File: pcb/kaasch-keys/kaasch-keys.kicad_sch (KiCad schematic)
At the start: 62 parts, among them SW1 SW_Push, SW10 SW_Push, SW11 SW_Push, SW12 SW_Push, SW13 SW_Push, SW14 SW_Push, SW15 SW_Push, SW16 SW_Push, SW17 SW_Push, SW18 SW_Push, SW19 SW_Push, SW2 SW_Push, SW20 SW_Push, SW21 SW_Push, SW22 SW_Push, SW23 SW_Push, SW24 SW_Push, SW25 SW_Push, SW26 SW_Push, SW27 SW_Push, SW28 SW_Push, SW29 SW_Push, SW3 SW_Push, SW30 SW_Push, SW4 SW_Push, SW5 SW_Push, SW6 SW_Push, SW7 SW_Push, SW8 SW_Push, SW9 SW_Push

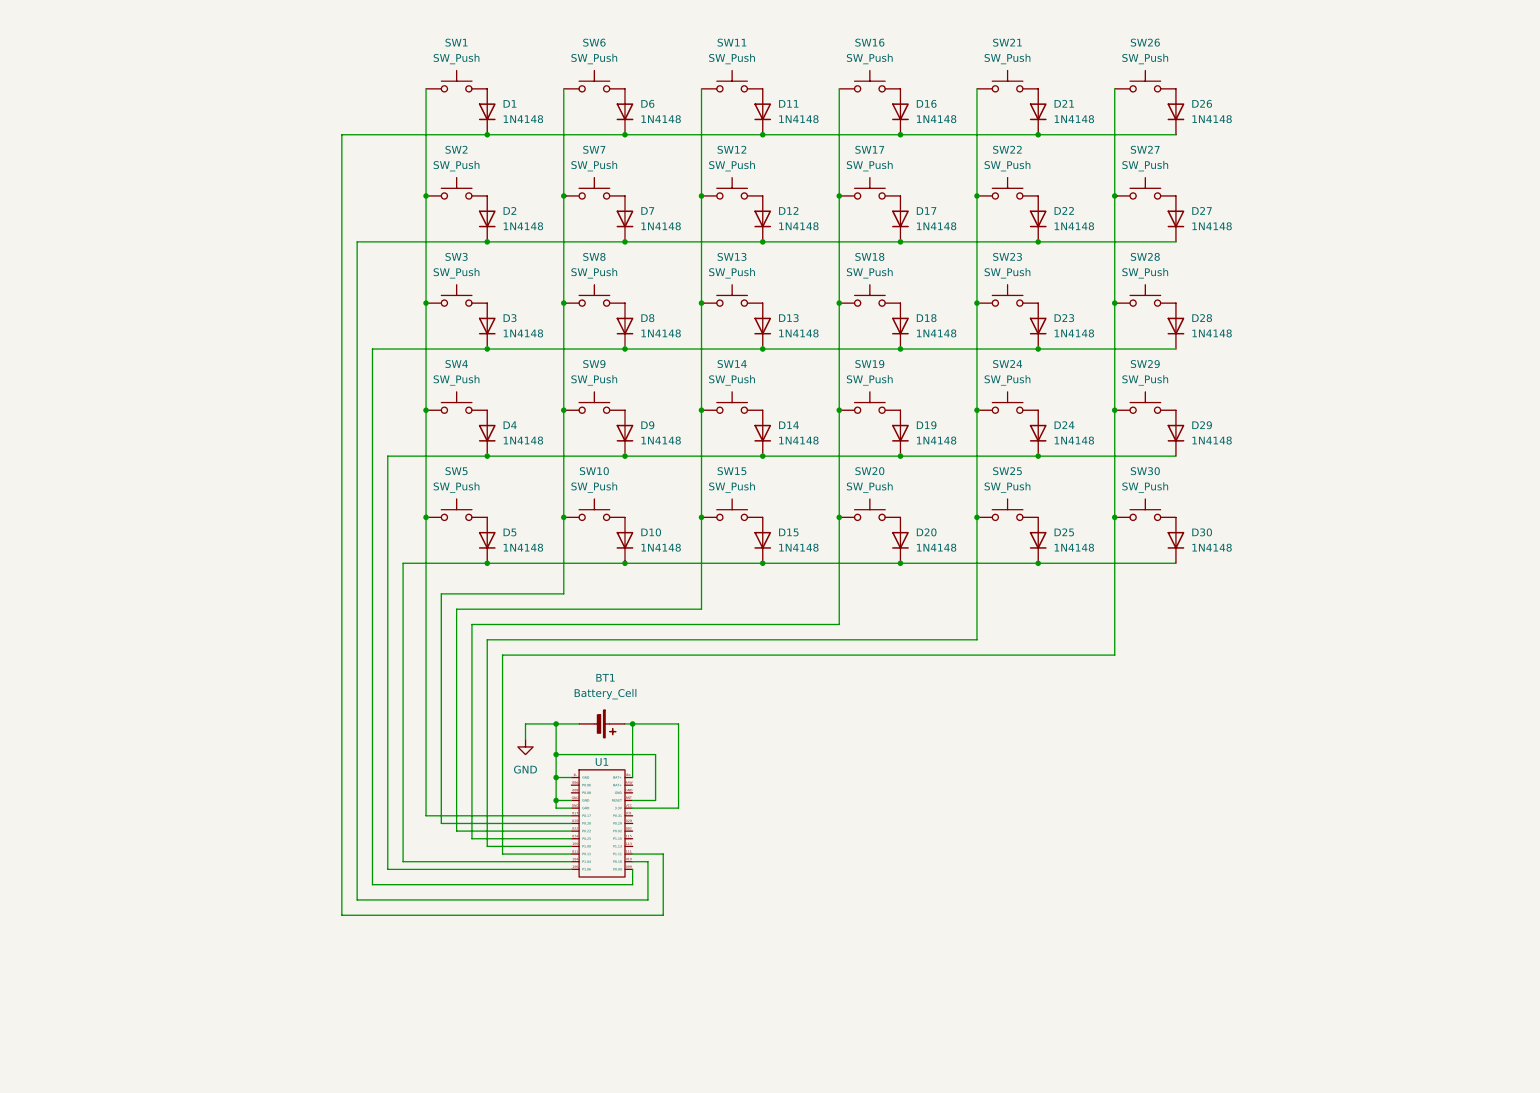
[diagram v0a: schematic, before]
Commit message: lets goo
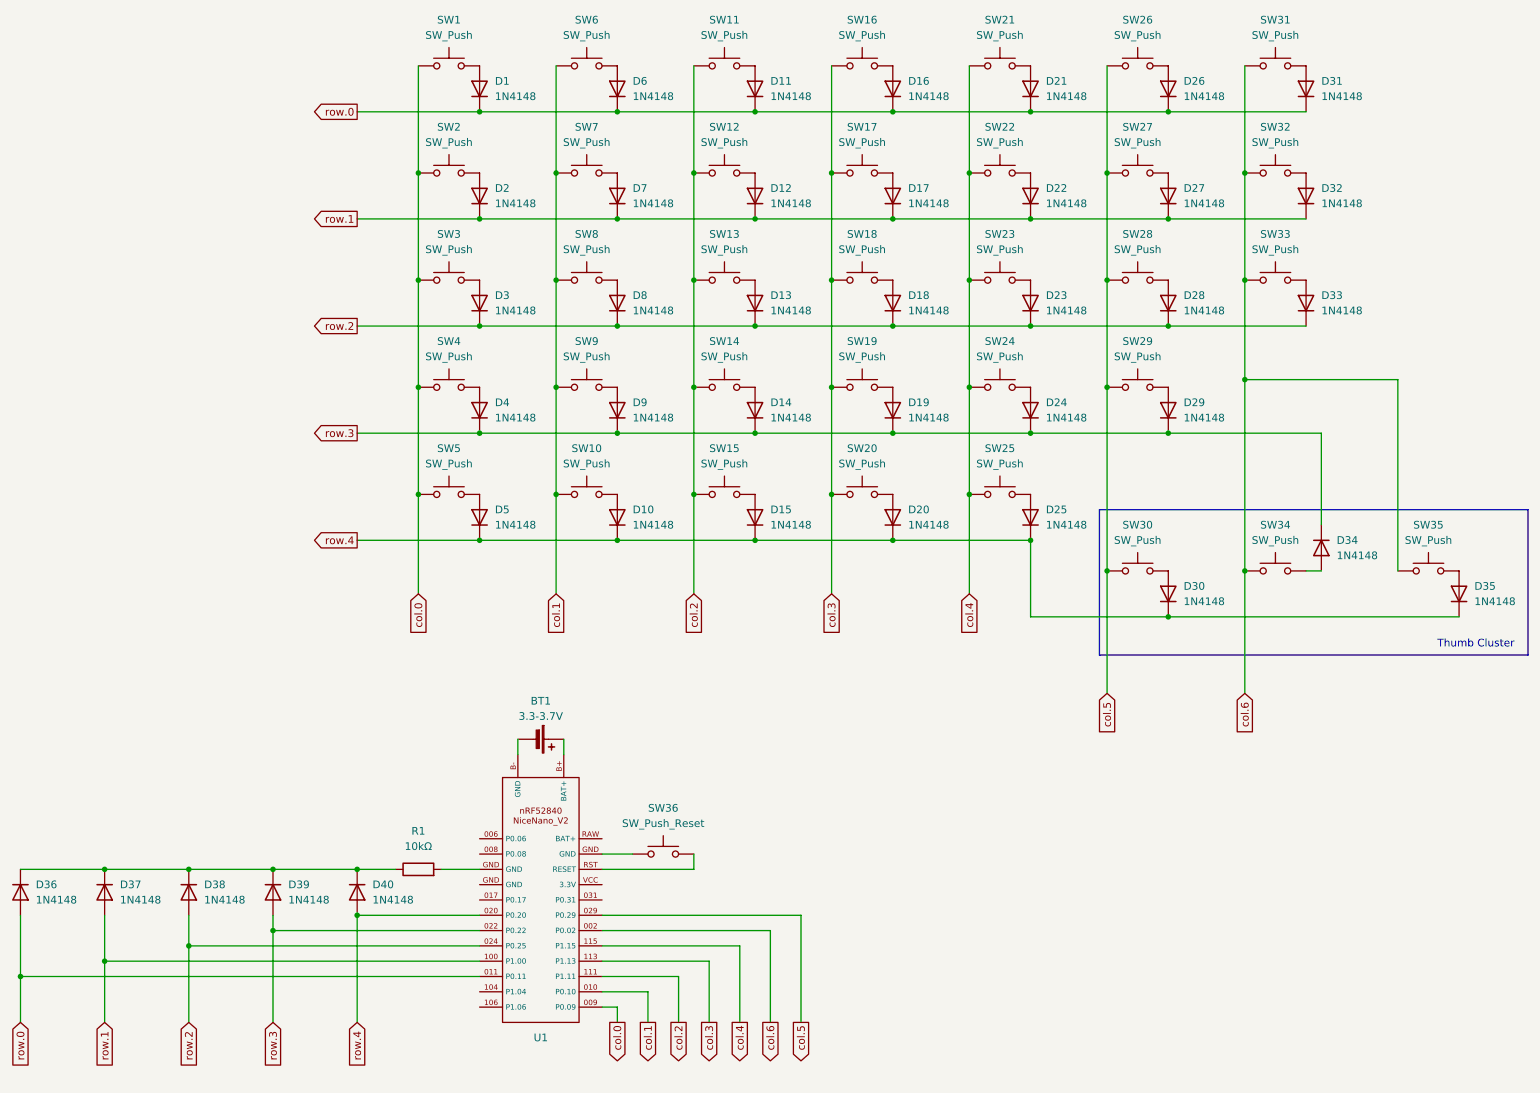
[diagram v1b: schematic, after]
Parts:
- added D31, D32, D33, D34, D35, D36, D37, D38, D39, D40: 1N4148, Diode_THT:D_DO-35_SOD27_P7.62mm_Horizontal, symbol Diode:1N4148
- added R1: 10kΩ, symbol Device:R
- added SW31, SW32, SW33, SW34, SW35: SW_Push, symbol Switch:SW_Push
- added SW36: SW_Push_Reset, symbol Switch:SW_Push
- BT1: value Battery_Cell -> 3.3-3.7V
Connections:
- net col.0: now reaches SW1.1, SW2.1, SW3.1, SW4.1, SW5.1
- net col.0: now also U1.009 (P0.09); no longer U1.017 (P0.17)
- net row.3: now reaches D14.1 (K), D19.1 (K), D24.1 (K), D29.1 (K), D4.1 (K), D9.1 (K)
- net row.3: now also U1.022 (P0.22), D34.1 (K), D39.2 (A); no longer U1.106 (P1.06)
- net row.4: now reaches D10.1 (K), D15.1 (K), D20.1 (K), D25.1 (K), D30.1 (K), D5.1 (K)
- net row.4: now also U1.020 (P0.20), D35.1 (K), D40.2 (A); no longer U1.104 (P1.04)
- net row.2: now reaches D13.1 (K), D18.1 (K), D23.1 (K), D28.1 (K), D3.1 (K), D8.1 (K)
- net row.2: now also U1.024 (P0.25), D33.1 (K), D38.2 (A); no longer U1.009 (P0.09)
- net col.2: now reaches SW11.1, SW12.1, SW13.1, SW14.1, SW15.1
- net col.2: now also U1.111 (P1.11); no longer U1.022 (P0.22)
- net row.1: now reaches D12.1 (K), D17.1 (K), D2.1 (K), D22.1 (K), D27.1 (K), D7.1 (K)
- net row.1: now also U1.100 (P1.00), D32.1 (K), D37.2 (A); no longer U1.010 (P0.10)
- net col.3: now reaches SW16.1, SW17.1, SW18.1, SW19.1, SW20.1
- net col.3: now also U1.113 (P1.13); no longer U1.024 (P0.25)
- net row.0: now reaches D1.1 (K), D11.1 (K), D16.1 (K), D21.1 (K), D26.1 (K), D6.1 (K)
- net row.0: now also U1.011 (P0.11), D31.1 (K), D36.2 (A); no longer U1.111 (P1.11)
- net col.4: now reaches SW21.1, SW22.1, SW23.1, SW24.1, SW25.1
- net col.4: now also U1.115 (P1.15); no longer U1.100 (P1.00)
- net col.1: now reaches SW10.1, SW6.1, SW7.1, SW8.1, SW9.1
- net col.1: now also U1.010 (P0.10); no longer U1.020 (P0.20)
- net col.6: now reaches U1.002 (P0.02)
- net col.6: now also SW31.1, SW32.1, SW33.1, SW34.1, SW35.1
- net col.5: now reaches SW26.1, SW27.1, SW28.1, SW29.1, SW30.1
- net col.5: now also U1.029 (P0.29); no longer U1.011 (P0.11)
- net at BT1.1 (+), U1.B+ (BAT+): no longer U1.VCC (3.3V)
- net at U1.GND: now also R1.2
- net GND: no longer names the net of BT1.2 (-), U1.B- (GND)
- net GND: no longer U1.GND, U1.RST (RESET)
- new net: D33.2 (A), SW33.2
- new net: D36.1 (K), D37.1 (K), D38.1 (K), D39.1 (K), D40.1 (K), R1.1
- new net: D35.2 (A), SW35.2
- new net: SW36.1, U1.GND
- new net: SW36.2, U1.RST (RESET)
- new net: D34.2 (A), SW34.2
- new net: D32.2 (A), SW32.2
- new net: D31.2 (A), SW31.2
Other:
- note added: "Thumb Cluster"
- moved on the sheet: D1, D10, D11, D12, D13, D14, D15, D16, D17, D18, D19, D2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
